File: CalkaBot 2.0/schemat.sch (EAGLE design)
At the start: 55 parts, among them IC1 TB6612FNG, IC2 LM339D, IC3 7806DT, Q1 16MHz, X1 MINI-USB-32005-301

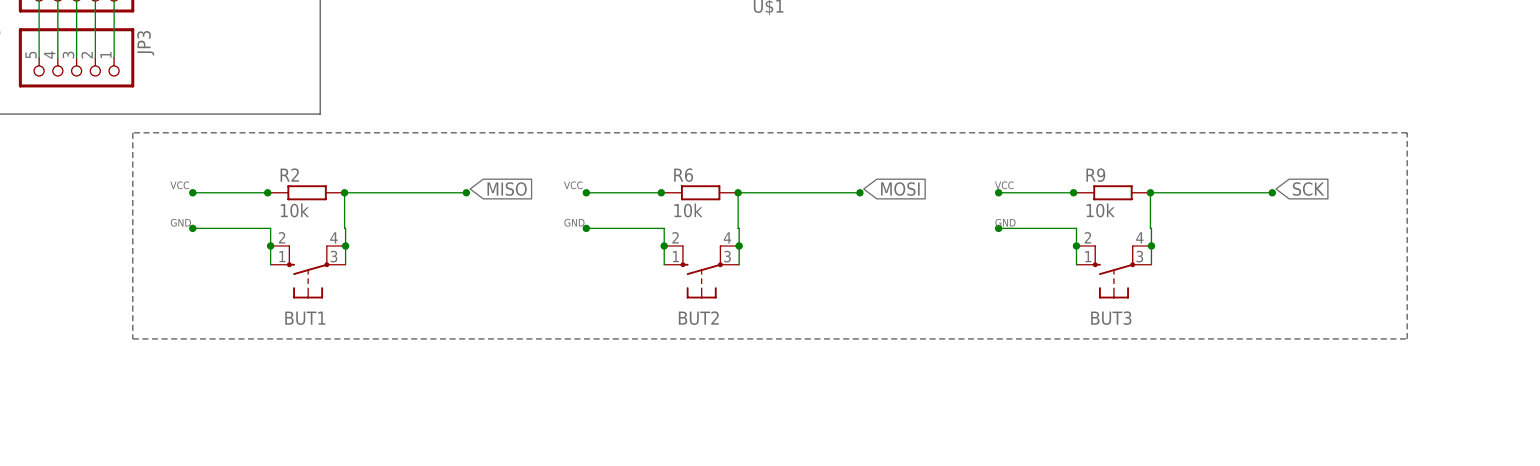
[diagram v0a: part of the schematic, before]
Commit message: zmiana przycisków
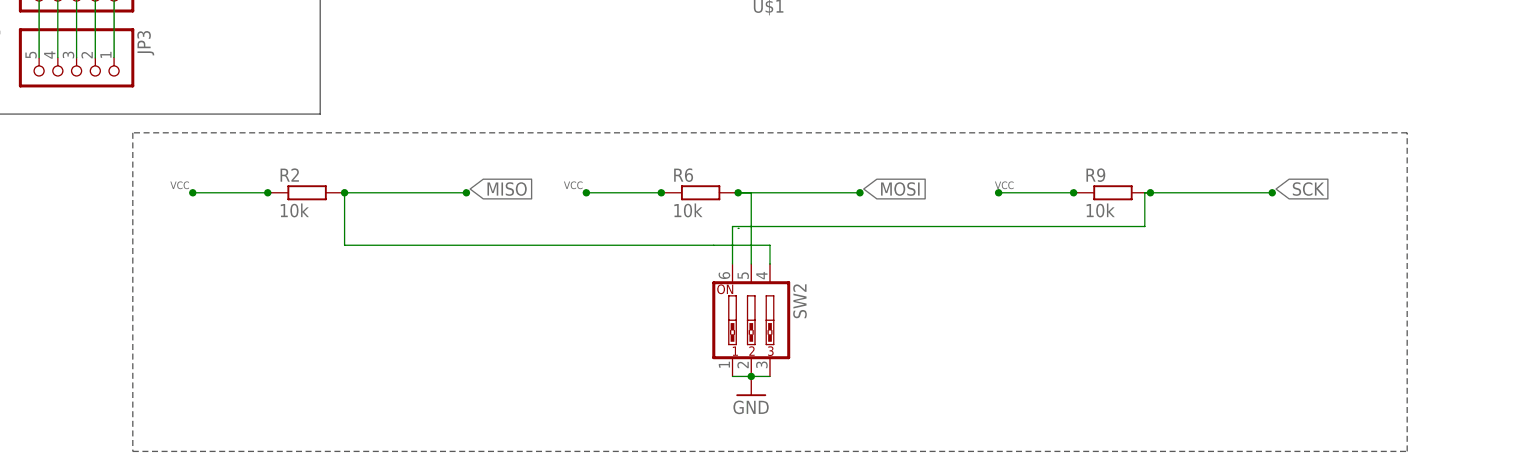
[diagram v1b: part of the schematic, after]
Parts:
- removed BUT1, BUT2, BUT3: (no value), switch-omron:10-XX
- added SW2: (no value), special:SW_DIP-3
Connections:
- net GND: now also SW2.1, SW2.2, SW2.3; no longer BUT1.S, BUT1.S1, BUT2.S, BUT2.S1, BUT3.S, BUT3.S1
- net MISO: now also SW2.4; no longer BUT1.P, BUT1.P1
- net MOSI: now also SW2.5; no longer BUT2.P, BUT2.P1
- net SCK: now also SW2.6; no longer BUT3.P, BUT3.P1
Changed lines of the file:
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@@
 <?xml version="1.0" encoding="utf-8"?>
 <!DOCTYPE eagle SYSTEM "eagle.dtd">
-<eagle version="8.6.0">
+<eagle version="9.1.3">
 <drawing>
 <settings>
@@
 <part name="GND4" library="supply1" library_urn="urn:adsk.eagle:library:371" deviceset="GND" device=""/>
 <part name="R2" library="rcl" library_urn="urn:adsk.eagle:library:334" deviceset="R-EU_" device="R0805" package3d_urn="urn:adsk.eagle:package:23553/2" value="10k"/>
-<part name="BUT1" library="switch-omron" library_urn="urn:adsk.eagle:library:377" deviceset="10-XX" device="" package3d_urn="urn:adsk.eagle:package:27496/1"/>
 <part name="X1" library="con-cypressindustries" library_urn="urn:adsk.eagle:library:138" deviceset="MINI-USB-" device="32005-301" package3d_urn="urn:adsk.eagle:package:6446/1"/>
 <part name="R6" library="rcl" library_urn="urn:adsk.eagle:library:334" deviceset="R-EU_" device="R0805" package3d_urn="urn:adsk.eagle:package:23553/2" value="10k"/>
-<part name="BUT2" library="switch-omron" library_urn="urn:adsk.eagle:library:377" deviceset="10-XX" device="" package3d_urn="urn:adsk.eagle:package:27496/1"/>
 <part name="R9" library="rcl" library_urn="urn:adsk.eagle:library:334" deviceset="R-EU_" device="R0805" package3d_urn="urn:adsk.eagle:package:23553/2" value="10k"/>
-<part name="BUT3" library="switch-omron" library_urn="urn:adsk.eagle:library:377" deviceset="10-XX" device="" package3d_urn="urn:adsk.eagle:package:27496/1"/>
 <part name="IC3" library="linear3" deviceset="78*" device="DT" technology="06"/>
 <part name="GND7" library="supply1" library_urn="urn:adsk.eagle:library:371" deviceset="GND" device=""/>
@@
 <part name="JP2" library="pinhead" library_urn="urn:adsk.eagle:library:325" deviceset="PINHD-1X5" device="" package3d_urn="urn:adsk.eagle:package:22469/2"/>
 <part name="JP3" library="pinhead" library_urn="urn:adsk.eagle:library:325" deviceset="PINHD-1X5" device="" package3d_urn="urn:adsk.eagle:package:22469/2"/>
+<part name="SW2" library="special" library_urn="urn:adsk.eagle:library:367" deviceset="SW_DIP-3" device="" package3d_urn="urn:adsk.eagle:package:26663/2"/>
+<part name="GND22" library="supply1" library_urn="urn:adsk.eagle:library:371" deviceset="GND" device=""/>
 </parts>
 <sheets>
@@
 <instance part="GND4" gate="1" x="70.866" y="69.85"/>
 <instance part="R2" gate="G$1" x="-88.138" y="-0.508"/>
-<instance part="BUT1" gate="1" x="-88" y="-10.26" rot="R90"/>
 <instance part="X1" gate="G$1" x="-149.86" y="43.18" rot="R180"/>
 <instance part="R6" gate="G$1" x="-34.798" y="-0.508"/>
-<instance part="BUT2" gate="1" x="-34.66" y="-10.26" rot="R90"/>
 <instance part="R9" gate="G$1" x="21.082" y="-0.508"/>
-<instance part="BUT3" gate="1" x="21.22" y="-10.26" rot="R90"/>
 <instance part="IC3" gate="A1" x="68.58" y="124.46"/>
 <instance part="GND7" gate="1" x="68.58" y="111.76"/>
@@
 <instance part="JP2" gate="A" x="-119.38" y="25.4" rot="R270"/>
 <instance part="JP3" gate="A" x="-119.38" y="15.24" rot="R270"/>
+<instance part="SW2" gate="A" x="-27.94" y="-17.78" rot="R270"/>
+<instance part="GND22" gate="1" x="-27.94" y="-27.94"/>
 </instances>
 <busses>
@@
 <bus name="B$3">
 <segment>
-<wire x1="-111.76" y1="7.62" x2="-111.76" y2="-20.32" width="0.762" layer="92" style="shortdash"/>
-<wire x1="-111.76" y1="-20.32" x2="60.96" y2="-20.32" width="0.762" layer="92" style="shortdash"/>
-<wire x1="60.96" y1="-20.32" x2="60.96" y2="7.62" width="0.762" layer="92" style="shortdash"/>
+<wire x1="-111.76" y1="7.62" x2="-111.76" y2="-35.56" width="0.762" layer="92" style="shortdash"/>
+<wire x1="-111.76" y1="-35.56" x2="60.96" y2="-35.56" width="0.762" layer="92" style="shortdash"/>
+<wire x1="60.96" y1="-35.56" x2="60.96" y2="7.62" width="0.762" layer="92" style="shortdash"/>
 <wire x1="60.96" y1="7.62" x2="-111.76" y2="7.62" width="0.762" layer="92" style="shortdash"/>
 </segment>
@@
 </segment>
 <segment>
-<wire x1="-93.08" y1="-5.334" x2="-103.632" y2="-5.334" width="0.1524" layer="91"/>
-<junction x="-103.632" y="-5.334"/>
-<pinref part="BUT1" gate="1" pin="S"/>
-<pinref part="BUT1" gate="1" pin="S1"/>
-<wire x1="-93.08" y1="-10.26" x2="-93.08" y2="-7.72" width="0.1524" layer="91"/>
-<wire x1="-93.08" y1="-7.72" x2="-93.08" y2="-5.334" width="0.1524" layer="91"/>
-<junction x="-93.08" y="-7.72"/>
-<label x="-106.68" y="-5.08" size="1.016" layer="95"/>
-</segment>
-<segment>
 <pinref part="IC3" gate="A1" pin="GND"/>
 <wire x1="68.58" y1="116.84" x2="68.58" y2="114.3" width="0.1524" layer="91"/>
@@
 <wire x1="55.88" y1="137.16" x2="55.88" y2="132.08" width="0.1524" layer="91"/>
 <pinref part="GND18" gate="1" pin="GND"/>
-</segment>
-<segment>
-<wire x1="16.14" y1="-5.334" x2="5.588" y2="-5.334" width="0.1524" layer="91"/>
-<junction x="5.588" y="-5.334"/>
-<pinref part="BUT3" gate="1" pin="S"/>
-<pinref part="BUT3" gate="1" pin="S1"/>
-<wire x1="16.14" y1="-10.26" x2="16.14" y2="-7.72" width="0.1524" layer="91"/>
-<wire x1="16.14" y1="-7.72" x2="16.14" y2="-5.334" width="0.1524" layer="91"/>
-<junction x="16.14" y="-7.72"/>
-<label x="5.08" y="-5.08" size="1.016" layer="95"/>
-</segment>
-<segment>
-<wire x1="-39.74" y1="-5.334" x2="-50.292" y2="-5.334" width="0.1524" layer="91"/>
-<junction x="-50.292" y="-5.334"/>
-<pinref part="BUT2" gate="1" pin="S"/>
-<pinref part="BUT2" gate="1" pin="S1"/>
-<wire x1="-39.74" y1="-10.26" x2="-39.74" y2="-7.72" width="0.1524" layer="91"/>
-<wire x1="-39.74" y1="-7.72" x2="-39.74" y2="-5.334" width="0.1524" layer="91"/>
-<junction x="-39.74" y="-7.72"/>
-<label x="-53.34" y="-5.08" size="1.016" layer="95"/>
 </segment>
 <segment>
@@
 <label x="-46" y="44.5" size="1.778" layer="95"/>
 </segment>
+<segment>
+<pinref part="SW2" gate="A" pin="1"/>
+<pinref part="SW2" gate="A" pin="2"/>
+<wire x1="-30.48" y1="-25.4" x2="-27.94" y2="-25.4" width="0.1524" layer="91"/>
+<pinref part="SW2" gate="A" pin="3"/>
+<wire x1="-25.4" y1="-25.4" x2="-27.94" y2="-25.4" width="0.1524" layer="91"/>
+<junction x="-27.94" y="-25.4"/>
+<pinref part="GND22" gate="1" pin="GND"/>
+</segment>
 </net>
 <net name="D-" class="0">
@@
 <wire x1="-83.058" y1="-0.508" x2="-66.548" y2="-0.508" width="0.1524" layer="91"/>
 <junction x="-66.548" y="-0.508"/>
+<label x="-66.04" y="0" size="1.778" layer="95" xref="yes"/>
+<wire x1="-83.058" y1="-0.508" x2="-83.058" y2="-7.62" width="0.1524" layer="91"/>
+<wire x1="-83.058" y1="-7.62" x2="-33.02" y2="-7.62" width="0.1524" layer="91"/>
 <junction x="-83.058" y="-0.508"/>
-<wire x1="-83.058" y1="-5.334" x2="-83.058" y2="-0.508" width="0.1524" layer="91"/>
-<pinref part="BUT1" gate="1" pin="P1"/>
-<wire x1="-82.92" y1="-7.72" x2="-82.92" y2="-5.334" width="0.1524" layer="91"/>
-<wire x1="-82.92" y1="-5.334" x2="-83.058" y2="-5.334" width="0.1524" layer="91"/>
-<pinref part="BUT1" gate="1" pin="P"/>
-<wire x1="-82.92" y1="-10.26" x2="-82.92" y2="-7.72" width="0.1524" layer="91"/>
-<junction x="-82.92" y="-7.72"/>
-<label x="-66.04" y="0" size="1.778" layer="95" xref="yes"/>
+<pinref part="SW2" gate="A" pin="4"/>
+<wire x1="-33.02" y1="-7.62" x2="-30.48" y2="-7.62" width="0.1524" layer="91"/>
+<wire x1="-25.4" y1="-10.16" x2="-25.4" y2="-7.62" width="0.1524" layer="91"/>
+<wire x1="-25.4" y1="-7.62" x2="-30.48" y2="-7.62" width="0.1524" layer="91"/>
 </segment>
 </net>
@@
 <wire x1="-29.718" y1="-0.508" x2="-13.208" y2="-0.508" width="0.1524" layer="91"/>
 <junction x="-13.208" y="-0.508"/>
+<label x="-12.7" y="0" size="1.778" layer="95" xref="yes"/>
 <junction x="-29.718" y="-0.508"/>
-<wire x1="-29.718" y1="-5.334" x2="-29.718" y2="-0.508" width="0.1524" layer="91"/>
-<pinref part="BUT2" gate="1" pin="P1"/>
-<wire x1="-29.58" y1="-7.72" x2="-29.58" y2="-5.334" width="0.1524" layer="91"/>
-<wire x1="-29.58" y1="-5.334" x2="-29.718" y2="-5.334" width="0.1524" layer="91"/>
-<pinref part="BUT2" gate="1" pin="P"/>
-<wire x1="-29.58" y1="-10.26" x2="-29.58" y2="-7.72" width="0.1524" layer="91"/>
-<junction x="-29.58" y="-7.72"/>
-<label x="-12.7" y="0" size="1.778" layer="95" xref="yes"/>
+<pinref part="SW2" gate="A" pin="5"/>
+<wire x1="-29.718" y1="-0.508" x2="-27.94" y2="-0.508" width="0.1524" layer="91"/>
+<wire x1="-27.94" y1="-0.508" x2="-27.94" y2="-10.16" width="0.1524" layer="91"/>
 </segment>
 </net>
@@
 <wire x1="26.162" y1="-0.508" x2="42.672" y2="-0.508" width="0.1524" layer="91"/>
 <junction x="42.672" y="-0.508"/>
+<label x="43.18" y="0" size="1.778" layer="95" xref="yes"/>
+<wire x1="26.162" y1="-0.508" x2="25.4" y2="-0.508" width="0.1524" layer="91"/>
+<wire x1="25.4" y1="-0.508" x2="25.4" y2="-5.08" width="0.1524" layer="91"/>
 <junction x="26.162" y="-0.508"/>
-<wire x1="26.162" y1="-5.334" x2="26.162" y2="-0.508" width="0.1524" layer="91"/>
-<pinref part="BUT3" gate="1" pin="P1"/>
-<wire x1="26.3" y1="-7.72" x2="26.3" y2="-5.334" width="0.1524" layer="91"/>
-<wire x1="26.3" y1="-5.334" x2="26.162" y2="-5.334" width="0.1524" layer="91"/>
-<pinref part="BUT3" gate="1" pin="P"/>
-<wire x1="26.3" y1="-10.26" x2="26.3" y2="-7.72" width="0.1524" layer="91"/>
-<junction x="26.3" y="-7.72"/>
-<label x="43.18" y="0" size="1.778" layer="95" xref="yes"/>
+<wire x1="25.4" y1="-5.08" x2="-30.48" y2="-5.08" width="0.1524" layer="91"/>
+<pinref part="SW2" gate="A" pin="6"/>
+<wire x1="-30.48" y1="-10.16" x2="-30.48" y2="-5.08" width="0.1524" layer="91"/>
 </segment>
 </net>
@@
 </segment>
 </net>
+<net name="N$10" class="0">
+<segment>
+<wire x1="-29.58" y1="-5.334" x2="-29.718" y2="-5.334" width="0.1524" layer="91"/>
+</segment>
+</net>
